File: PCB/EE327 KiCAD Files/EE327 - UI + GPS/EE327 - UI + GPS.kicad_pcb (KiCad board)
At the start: 4 copper layers, 49.9 x 49.9 mm, 18 parts, among them J1 Conn_01x09_Socket, J2 Conn_01x14_Socket, J3 Conn_01x06_Pin, J4 Conn_01x04_Socket, J5 Conn_01x02_Socket, SW1 SW_Push, SW2 SW_Push, U1 ESP32-WROOM-32E-N4, U3 LDL1117S30R

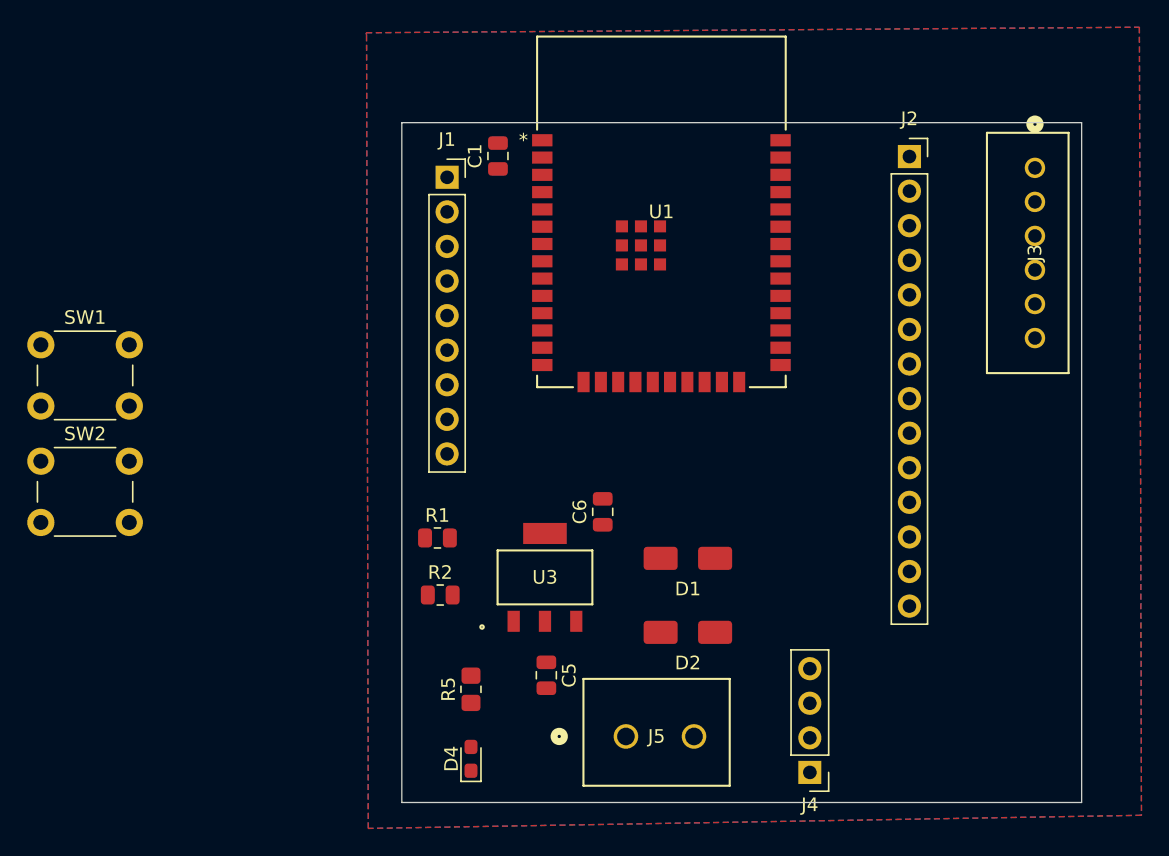
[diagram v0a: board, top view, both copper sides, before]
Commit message: PCB routing started
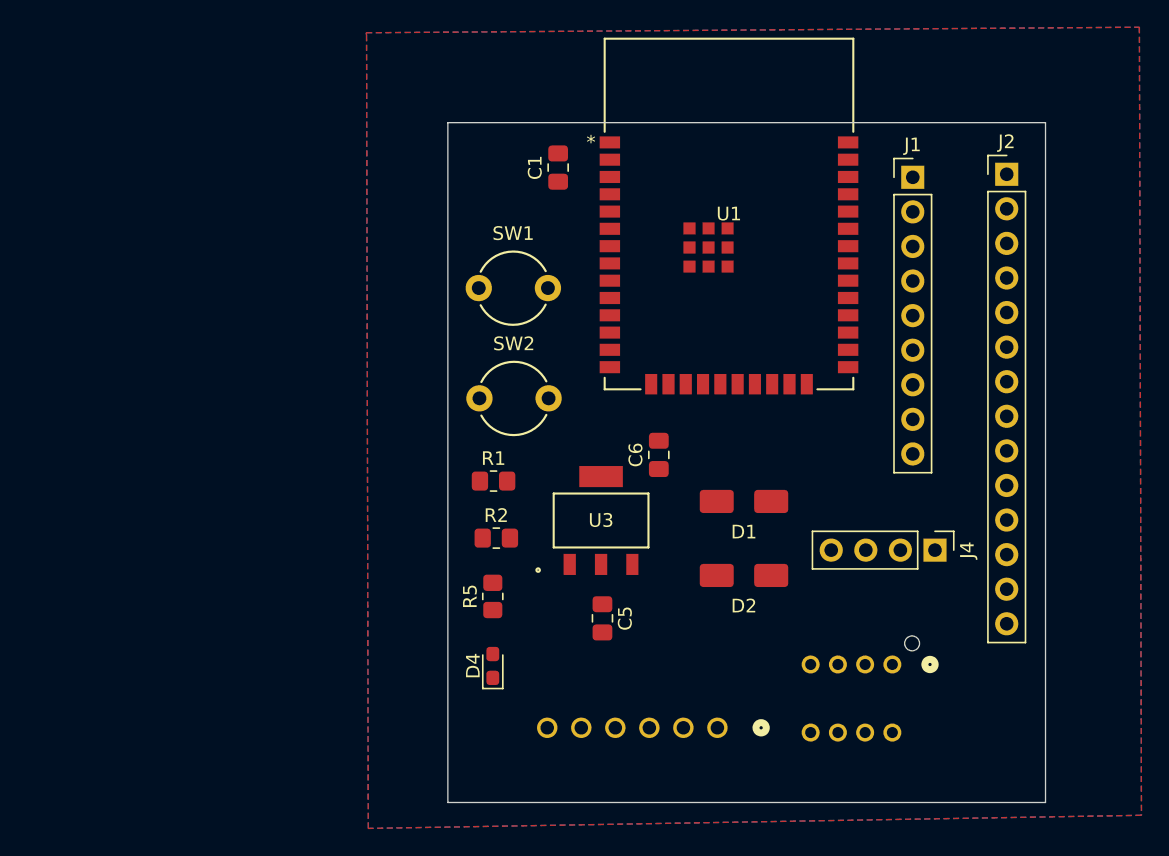
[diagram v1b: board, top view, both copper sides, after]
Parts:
- C1: value C -> 0.1uF; footprint Capacitor_SMD:C_0805_2012Metric -> Capacitor_SMD:C_0805_2012Metric_Pad1.18x1.45mm_HandSolder
- C5, C6: footprint Capacitor_SMD:C_0805_2012Metric -> Capacitor_SMD:C_0805_2012Metric_Pad1.18x1.45mm_HandSolder
- J1: footprint Connector_PinSocket_2.54mm:PinSocket_1x09_P2.54mm_Vertical -> Connector_PinHeader_2.54mm:PinHeader_1x09_P2.54mm_Vertical
- J2: footprint Connector_PinSocket_2.54mm:PinSocket_1x14_P2.54mm_Vertical -> Connector_PinHeader_2.54mm:PinHeader_1x14_P2.54mm_Vertical
- J3: moved to B.Cu
- J5: value Conn_01x02_Socket -> Conn_01x08_Socket; footprint EE327_Symbols:screw terminal -> EE327_Symbols:CONN_B08B-PNDZS-1_JST; moved to B.Cu
- R1, R2: footprint Resistor_SMD:R_0805_2012Metric -> Resistor_SMD:R_0805_2012Metric_Pad1.20x1.40mm_HandSolder
- SW1, SW2: footprint Button_Switch_THT:SW_PUSH_6mm -> EE327_Symbols:pushbutton
- moved J3 47.3 mm to (146.5, 127.0), turned to 0 degrees
- moved SW2 35.1 mm to (131.6, 102.8)
- moved SW1 35.0 mm to (131.5, 94.8)
- moved J1 34.2 mm to (160.8, 86.6)
- moved J5 20.3 mm to (159.3, 122.4), turned to 180 degrees
- moved J4 18.7 mm to (162.5, 114.0), turned to -90 degrees
- moved J2 7.26 mm to (167.8, 86.4)
- moved D4 7.01 mm to (130.0, 122.5)
- moved R5 7.01 mm to (130.0, 117.4)
- moved R2 5.87 mm to (130.3, 113.1)
- moved C5 5.87 mm to (138.1, 119.0)
- moved C6 5.87 mm to (142.2, 107.0)
- moved D1 5.87 mm to (148.4, 113.2)
- moved D2 5.87 mm to (148.4, 118.6)
- moved R1 5.87 mm to (130.1, 108.9)
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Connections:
- J2 pad 8: unconnected-(J2-Pin_8-Pad8) -> +3.3V
- J5 pad 1: GND -> /Terminal_5V
- J5 pad 2: /Terminal_5V -> GND
- U1 pad 10: unconnected-(U1-IO25-Pad10) -> /PMIC_~{INT}
- U1 pad 11: unconnected-(U1-IO26-Pad11) -> /PMIC_STAT1
- U1 pad 12: unconnected-(U1-IO27-Pad12) -> /PMIC_STAT2
- U1 pad 13: unconnected-(U1-IO14-Pad13) -> /PMIC_~{PG}
- U1 pad 15: unconnected-(U1-GND-Pad15) -> GND
- U1 pad 30: unconnected-(U1-IO18-Pad30) -> /TFT_SCK
- U1 pad 31: /TFT_SCK -> unconnected-(U1-IO19-Pad31)
- U1 pad 33: unconnected-(U1-IO21-Pad33) -> /SDA
- U1 pad 36: unconnected-(U1-IO22-Pad36) -> /SCL
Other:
- board size 49.9 x 49.9 mm -> 43.9 x 49.9 mm

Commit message: pcb done?
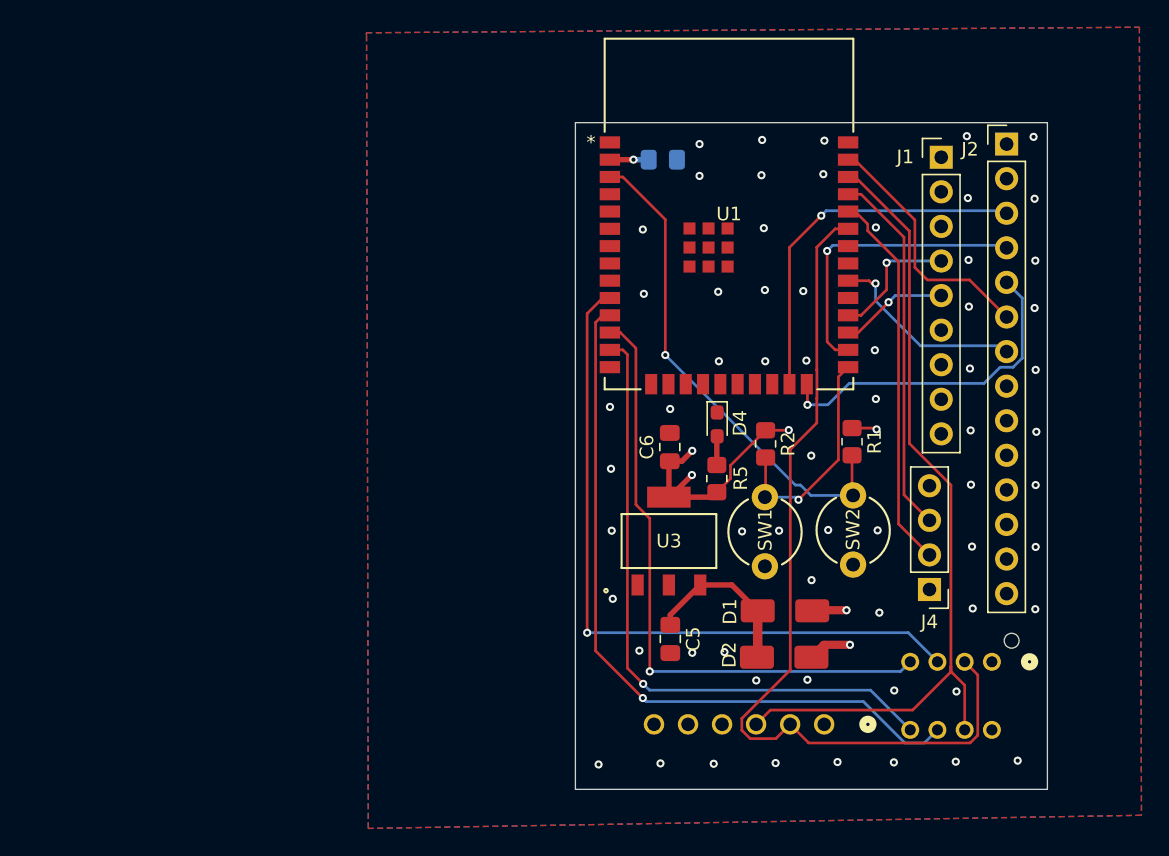
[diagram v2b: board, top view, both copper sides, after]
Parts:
- C1: moved to B.Cu
- moved SW1 30.6 mm to (156.5, 112.5), turned to 90 degrees
- moved R1 26.5 mm to (156.4, 106.0), turned to -90 degrees
- moved D4 24.2 mm to (146.5, 104.8), turned to -90 degrees
- moved R2 21.0 mm to (150.0, 106.2), turned to -90 degrees
- moved SW2 20.9 mm to (150.0, 112.6), turned to 90 degrees
- moved R5 18.6 mm to (146.5, 108.7)
- moved D1 8.58 mm to (151.5, 121.2)
- moved J3 7.85 mm to (154.3, 126.8)
- moved C1 7.71 mm to (142.5, 85.3), turned to 0 degrees
- moved J5 7.31 mm to (166.7, 122.2)
- moved D2 6.69 mm to (151.4, 124.6)
- moved C5 5.21 mm to (143.0, 120.5)
- moved U3 5.21 mm to (142.9, 113.3)
- moved J4 2.92 mm to (162.1, 116.9), turned to 180 degrees
- moved J1 2.56 mm to (162.9, 85.1)
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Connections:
- C6 pad 1: +3V3 -> +3.3V
- R1 pad 2: GND -> /ESP_RST
- R2 pad 2: GND -> /BOOT
- R5 pad 1: +3V3 -> +3.3V
- U3 pad 4: +3V3 -> +3.3V
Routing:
- net +3.3V: track 0.00 -> 115.6 mm, vias 0 -> 5
- net /SDA: track 0.00 -> 65.3 mm
- net /SCL: track 0.00 -> 60.8 mm
- net /PMIC_STAT1: track 0.00 -> 53.7 mm, vias 0 -> 1
- net /PMIC_~{INT}: track 0.00 -> 52.2 mm, vias 0 -> 1
- net /PMIC_~{PG}: track 0.00 -> 47.1 mm, vias 0 -> 1
- net /PMIC_STAT2: track 0.00 -> 46.0 mm, vias 0 -> 1
- net /ESP_RST: track 0.00 -> 36.4 mm, vias 0 -> 1
- net /RX0: track 0.00 -> 28.0 mm
- net /TFT_CS: track 0.00 -> 27.2 mm, vias 0 -> 1
- net /TX0: track 0.00 -> 27.0 mm
- net /TFT_DC: track 0.00 -> 24.8 mm, vias 0 -> 1
- net /TFT_RST: track 0.00 -> 21.9 mm, vias 0 -> 1
- net /TFT_MOSI: track 0.00 -> 18.5 mm
- net /BOOT: track 0.00 -> 16.7 mm, vias 0 -> 1
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- added copper zone on In2.Cu, net GND
- removed copper zone on In2.Cu, net +3.3V
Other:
- board size 43.9 x 49.9 mm -> 34.7 x 49 mm
- board text added: "CycloSense AG/OK/JP 2026 EE 327"
- board text added: "SW2"
